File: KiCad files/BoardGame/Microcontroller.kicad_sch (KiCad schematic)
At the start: 11 parts

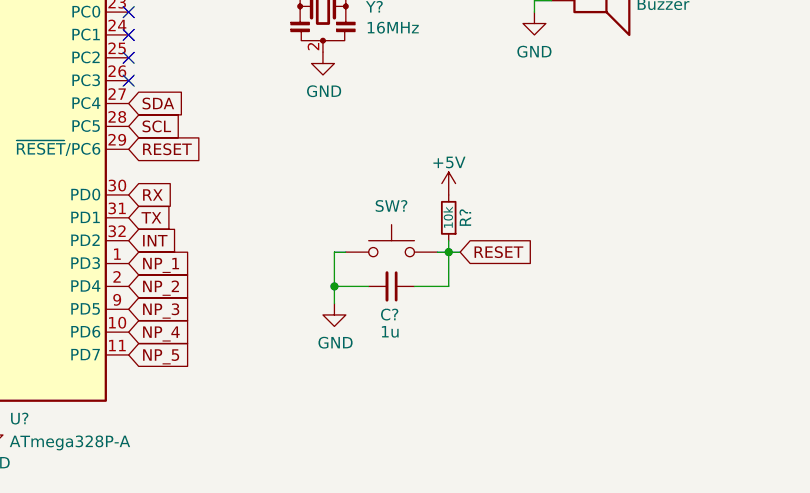
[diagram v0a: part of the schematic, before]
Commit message: update
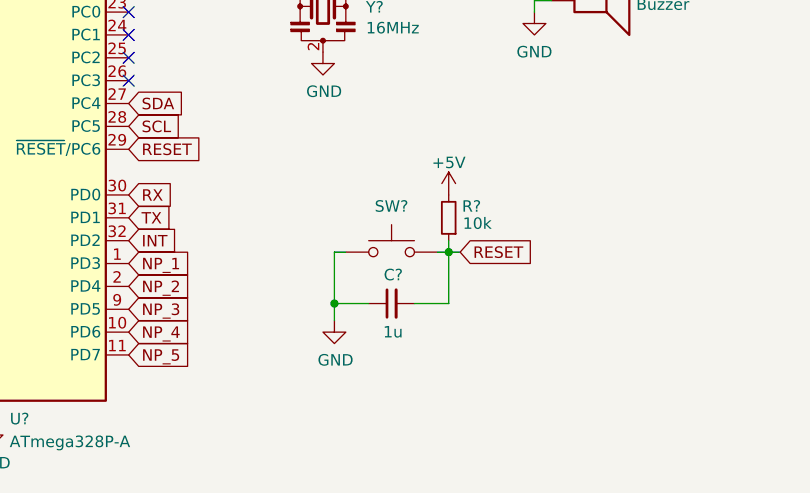
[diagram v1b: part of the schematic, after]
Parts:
- removed C? (x2): 100n, symbol Device:C_Small
- removed C?: 1u, symbol Device:C_Small
- added C? (x2): 100n, Capacitor_SMD:C_0603_1608Metric, symbol Device:C_Small
- added C?: 1u, Capacitor_SMD:C_0603_1608Metric, symbol Device:C_Small
- C?: footprint (none) -> Capacitor_SMD:C_0603_1608Metric; Basic/Extended Basic -> (none); JLCPCB Part # C49678 -> (none); U labosu? Da -> (none)
- L?: Basic/Extended Extended -> (none); JLCPCB Part # C279941 -> (none); U labosu? Ne -> (none)
- R?: footprint (none) -> Resistor_SMD:R_0603_1608Metric; Basic/Extended Basic -> (none); JLCPCB Part # C17414 -> (none); U labosu? Da -> (none)
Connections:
- net +5V: now also C?.1
- net GND: now also C?.1, C?.2, C?.2
- net RESET: now also C?.2
- net at L?.2, U?.18 (AVCC): now also C?.1
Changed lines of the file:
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@@
   (junction (at 154.305 62.23) (diameter 0) (color 0 0 0 0)
   )
-  (junction (at 170.815 128.905) (diameter 0) (color 0 0 0 0)
+  (junction (at 170.815 130.81) (diameter 0) (color 0 0 0 0)
   )
   (junction (at 123.19 62.23) (diameter 0) (color 0 0 0 0)
@@
     (stroke (width 0) (type default) (color 0 0 0 0))
   )
-  (wire (pts (xy 174.625 128.905) (xy 170.815 128.905))
-    (stroke (width 0) (type default) (color 0 0 0 0))
-  )
   (wire (pts (xy 135.255 67.945) (xy 135.255 62.23))
     (stroke (width 0) (type default) (color 0 0 0 0))
@@
     (stroke (width 0) (type default) (color 0 0 0 0))
   )
-  (wire (pts (xy 170.815 130.81) (xy 170.815 128.905))
+  (wire (pts (xy 179.705 130.81) (xy 183.515 130.81))
+    (stroke (width 0) (type default) (color 0 0 0 0))
+  )
+  (wire (pts (xy 170.815 132.715) (xy 170.815 130.81))
     (stroke (width 0) (type default) (color 0 0 0 0))
   )
@@
     (stroke (width 0) (type default) (color 0 0 0 0))
   )
-  (wire (pts (xy 179.705 128.905) (xy 183.515 128.905))
-    (stroke (width 0) (type default) (color 0 0 0 0))
-  )
   (wire (pts (xy 132.715 62.23) (xy 132.715 67.945))
     (stroke (width 0) (type default) (color 0 0 0 0))
@@
     (stroke (width 0) (type default) (color 0 0 0 0))
   )
-  (wire (pts (xy 183.515 128.905) (xy 183.515 125.095))
-    (stroke (width 0) (type default) (color 0 0 0 0))
-  )
   (wire (pts (xy 135.255 62.23) (xy 140.335 62.23))
     (stroke (width 0) (type default) (color 0 0 0 0))
@@
     (stroke (width 0) (type default) (color 0 0 0 0))
   )
-  (wire (pts (xy 170.815 128.905) (xy 170.815 125.095))
+  (wire (pts (xy 183.515 125.095) (xy 183.515 130.81))
+    (stroke (width 0) (type default) (color 0 0 0 0))
+  )
+  (wire (pts (xy 170.815 130.81) (xy 174.625 130.81))
+    (stroke (width 0) (type default) (color 0 0 0 0))
+  )
+  (wire (pts (xy 170.815 125.095) (xy 170.815 130.81))
     (stroke (width 0) (type default) (color 0 0 0 0))
   )
@@
   (symbol (lib_id "Device:R_Small") (at 183.515 121.285 180) (unit 1)
     (in_bom yes) (on_board yes)
-    (property "Reference" "R?" (id 0) (at 185.42 121.285 90))
-    (property "Value" "10k" (id 1) (at 183.515 121.285 90)
-      (effects (font (size 0.9906 0.9906)))
-    )
-    (property "Footprint" "" (id 2) (at 183.515 121.285 0)
+    (property "Reference" "R?" (id 0) (at 186.055 120.015 0))
+    (property "Value" "10k" (id 1) (at 186.69 121.92 0))
+    (property "Footprint" "Resistor_SMD:R_0603_1608Metric" (id 2) (at 183.515 121.285 0)
       (effects (font (size 1.27 1.27)) hide)
     )
     (property "Datasheet" "~" (id 3) (at 183.515 121.285 0)
-      (effects (font (size 1.27 1.27)) hide)
-    )
-    (property "Basic/Extended" "Basic" (id 4) (at 183.515 121.285 0)
-      (effects (font (size 1.27 1.27)) hide)
-    )
-    (property "JLCPCB Part #" "C17414" (id 5) (at 183.515 121.285 0)
-      (effects (font (size 1.27 1.27)) hide)
-    )
-    (property "U labosu?" "Da" (id 6) (at 183.515 121.285 0)
       (effects (font (size 1.27 1.27)) hide)
     )
@@
       (effects (font (size 1.27 1.27)) (justify left))
     )
-    (property "Footprint" "" (id 2) (at 90.805 66.04 0)
+    (property "Footprint" "Capacitor_SMD:C_0603_1608Metric" (id 2) (at 90.805 66.04 0)
       (effects (font (size 1.27 1.27)) hide)
     )
@@
       (effects (font (size 1.27 1.27)) hide)
     )
-    (property "Basic/Extended" "Basic" (id 4) (at 90.805 66.04 0)
-      (effects (font (size 1.27 1.27)) hide)
-    )
-    (property "JLCPCB Part #" "C49678" (id 5) (at 90.805 66.04 0)
-      (effects (font (size 1.27 1.27)) hide)
-    )
-    (property "U labosu?" "Da" (id 6) (at 90.805 66.04 0)
-      (effects (font (size 1.27 1.27)) hide)
-    )
-    (pin "1")
-    (pin "2")
-  )
-  (symbol (lib_id "power:GND") (at 170.815 130.81 0) (unit 1)
-    (in_bom yes) (on_board yes)
-    (property "Reference" "#PWR?" (id 0) (at 170.815 137.16 0)
-      (effects (font (size 1.27 1.27)) hide)
-    )
-    (property "Value" "GND" (id 1) (at 170.942 135.2042 0))
-    (property "Footprint" "" (id 2) (at 170.815 130.81 0)
-      (effects (font (size 1.27 1.27)) hide)
-    )
-    (property "Datasheet" "" (id 3) (at 170.815 130.81 0)
+    (pin "1")
+    (pin "2")
+  )
+  (symbol (lib_id "power:GND") (at 170.815 132.715 0) (unit 1)
+    (in_bom yes) (on_board yes)
+    (property "Reference" "#PWR?" (id 0) (at 170.815 139.065 0)
+      (effects (font (size 1.27 1.27)) hide)
+    )
+    (property "Value" "GND" (id 1) (at 170.942 137.1092 0))
+    (property "Footprint" "" (id 2) (at 170.815 132.715 0)
+      (effects (font (size 1.27 1.27)) hide)
+    )
+    (property "Datasheet" "" (id 3) (at 170.815 132.715 0)
       (effects (font (size 1.27 1.27)) hide)
     )
@@
       (effects (font (size 1.27 1.27)) (justify left))
     )
-    (property "Footprint" "" (id 2) (at 154.305 67.31 0)
+    (property "Footprint" "Capacitor_SMD:C_0603_1608Metric" (id 2) (at 154.305 67.31 0)
       (effects (font (size 1.27 1.27)) hide)
     )
     (property "Datasheet" "~" (id 3) (at 154.305 67.31 0)
-      (effects (font (size 1.27 1.27)) hide)
-    )
-    (property "Basic/Extended" "Basic" (id 4) (at 154.305 67.31 0)
-      (effects (font (size 1.27 1.27)) hide)
-    )
-    (property "JLCPCB Part #" "C49678" (id 5) (at 154.305 67.31 0)
-      (effects (font (size 1.27 1.27)) hide)
-    )
-    (property "U labosu?" "Da" (id 6) (at 154.305 67.31 0)
-      (effects (font (size 1.27 1.27)) hide)
-    )
-    (pin "1")
-    (pin "2")
-  )
-  (symbol (lib_id "Device:C_Small") (at 177.165 128.905 270) (unit 1)
-    (in_bom yes) (on_board yes)
-    (property "Reference" "C?" (id 0) (at 175.895 132.08 90)
-      (effects (font (size 1.27 1.27)) (justify left))
-    )
-    (property "Value" "1u" (id 1) (at 175.895 133.985 90)
-      (effects (font (size 1.27 1.27)) (justify left))
-    )
-    (property "Footprint" "" (id 2) (at 177.165 128.905 0)
-      (effects (font (size 1.27 1.27)) hide)
-    )
-    (property "Datasheet" "~" (id 3) (at 177.165 128.905 0)
-      (effects (font (size 1.27 1.27)) hide)
-    )
-    (property "Basic/Extended" "Basic" (id 4) (at 177.165 128.905 0)
-      (effects (font (size 1.27 1.27)) hide)
-    )
-    (property "JLCPCB Part #" "C28323" (id 5) (at 177.165 128.905 0)
-      (effects (font (size 1.27 1.27)) hide)
-    )
-    (property "U labosu?" "Da" (id 6) (at 177.165 128.905 0)
       (effects (font (size 1.27 1.27)) hide)
     )
@@
     (pin "1")
   )
-  (symbol (lib_id "Device:C_Small") (at 105.41 82.55 0) (unit 1)
-    (in_bom yes) (on_board yes)
-    (property "Reference" "C?" (id 0) (at 107.7468 81.3816 0)
-      (effects (font (size 1.27 1.27)) (justify left))
-    )
-    (property "Value" "100n" (id 1) (at 107.7468 83.693 0)
-      (effects (font (size 1.27 1.27)) (justify left))
-    )
-    (property "Footprint" "" (id 2) (at 105.41 82.55 0)
-      (effects (font (size 1.27 1.27)) hide)
-    )
-    (property "Datasheet" "~" (id 3) (at 105.41 82.55 0)
-      (effects (font (size 1.27 1.27)) hide)
-    )
-    (property "Basic/Extended" "Basic" (id 4) (at 105.41 82.55 0)
-      (effects (font (size 1.27 1.27)) hide)
-    )
-    (property "JLCPCB Part #" "C49678" (id 5) (at 105.41 82.55 0)
-      (effects (font (size 1.27 1.27)) hide)
-    )
-    (property "U labosu?" "Da" (id 6) (at 105.41 82.55 0)
-      (effects (font (size 1.27 1.27)) hide)
-    )
-    (pin "1")
-    (pin "2")
-  )
   (symbol (lib_id "power:+5V") (at 154.305 52.07 0) (unit 1)
     (in_bom yes) (on_board yes) (fields_autoplaced)
@@
     (pin "1")
   )
+  (symbol (lib_id "Device:C_Small") (at 177.165 130.81 90) (unit 1)
+    (in_bom yes) (on_board yes)
+    (property "Reference" "C?" (id 0) (at 178.435 127.635 90)
+      (effects (font (size 1.27 1.27)) (justify left))
+    )
+    (property "Value" "1u" (id 1) (at 178.435 133.985 90)
+      (effects (font (size 1.27 1.27)) (justify left))
+    )
+    (property "Footprint" "Capacitor_SMD:C_0603_1608Metric" (id 2) (at 177.165 130.81 0)
+      (effects (font (size 1.27 1.27)) hide)
+    )
+    (property "Datasheet" "~" (id 3) (at 177.165 130.81 0)
+      (effects (font (size 1.27 1.27)) hide)
+    )
+    (pin "1")
+    (pin "2")
+  )
   (symbol (lib_id "power:+5V") (at 183.515 118.745 0) (unit 1)
     (in_bom yes) (on_board yes) (fields_autoplaced)
@@
       (effects (font (size 1.27 1.27)) hide)
     )
-    (property "Basic/Extended" "Extended" (id 4) (at 154.305 56.515 0)
-      (effects (font (size 1.27 1.27)) hide)
-    )
-    (property "JLCPCB Part #" "C279941" (id 5) (at 154.305 56.515 0)
-      (effects (font (size 1.27 1.27)) hide)
-    )
-    (property "U labosu?" "Ne" (id 6) (at 154.305 56.515 0)
-      (effects (font (size 1.27 1.27)) hide)
-    )
     (pin "1")
     (pin "2")
@@
     (pin "1")
   )
+  (symbol (lib_id "Device:C_Small") (at 105.41 82.55 0) (unit 1)
+    (in_bom yes) (on_board yes)
+    (property "Reference" "C?" (id 0) (at 107.7468 81.3816 0)
+      (effects (font (size 1.27 1.27)) (justify left))
+    )
+    (property "Value" "100n" (id 1) (at 107.7468 83.693 0)
+      (effects (font (size 1.27 1.27)) (justify left))
+    )
+    (property "Footprint" "Capacitor_SMD:C_0603_1608Metric" (id 2) (at 105.41 82.55 0)
+      (effects (font (size 1.27 1.27)) hide)
+    )
+    (property "Datasheet" "~" (id 3) (at 105.41 82.55 0)
+      (effects (font (size 1.27 1.27)) hide)
+    )
+    (pin "1")
+    (pin "2")
+  )
   (symbol (lib_id "Connector_Generic:Conn_02x03_Odd_Even") (at 207.01 63.5 0) (unit 1)
